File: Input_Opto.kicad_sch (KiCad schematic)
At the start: 9 parts, among them U1 TCMT4100

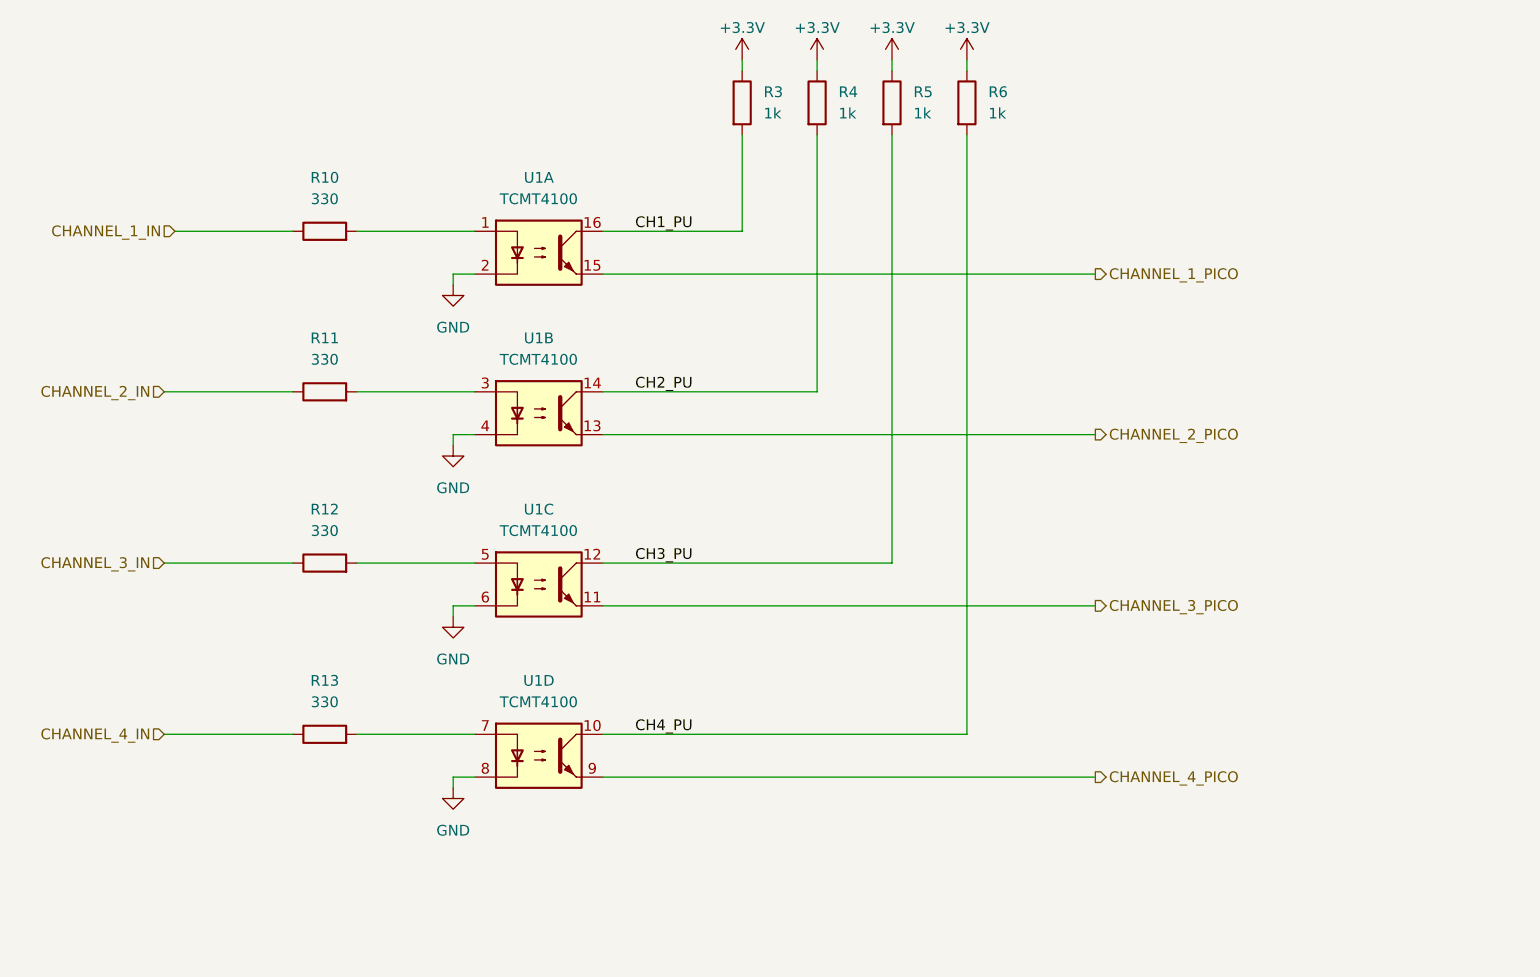
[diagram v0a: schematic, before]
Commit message: Letzte Changes
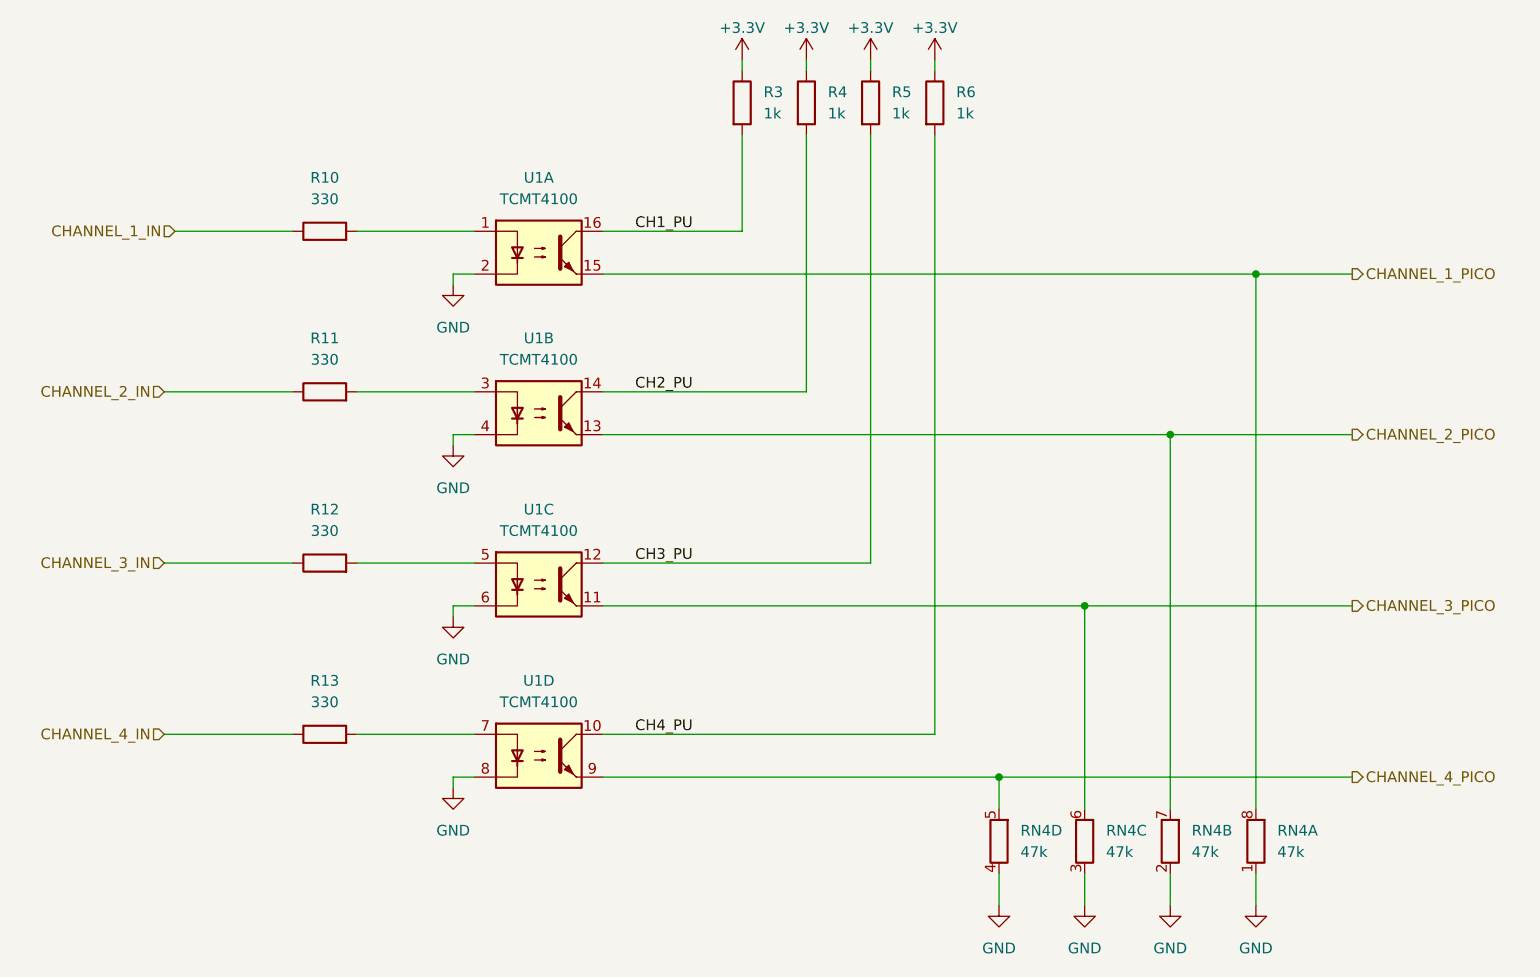
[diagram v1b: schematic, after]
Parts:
- added RN4: 47k, Resistor_SMD:R_Array_Convex_4x0603, symbol Device:R_Pack04_Split
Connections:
- net CHANNEL_1_PICO: now also RN4.8 (R1.2)
- net CHANNEL_2_PICO: now also RN4.7 (R2.2)
- net CHANNEL_3_PICO: now also RN4.6 (R3.2)
- net CHANNEL_4_PICO: now also RN4.5 (R4.2)
- net GND: now also RN4.1 (R1.1), RN4.2 (R2.1), RN4.3 (R3.1), RN4.4 (R4.1)
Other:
- moved on the sheet: R4, R5, R6
